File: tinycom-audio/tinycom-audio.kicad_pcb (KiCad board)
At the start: 2 copper layers, 45.2 x 45.2 mm, 73 parts, among them J1 MICRO_SD_HINGE, P1 CONN_02X10, P2 CONN_02X10, P4 USB_OTG, U1 SY8008BAAC, U2 AXP209, U3 SY8008BAAC, U4 RTL8188, U5 rainsun-antenna, U6 admp411, U7 admp411

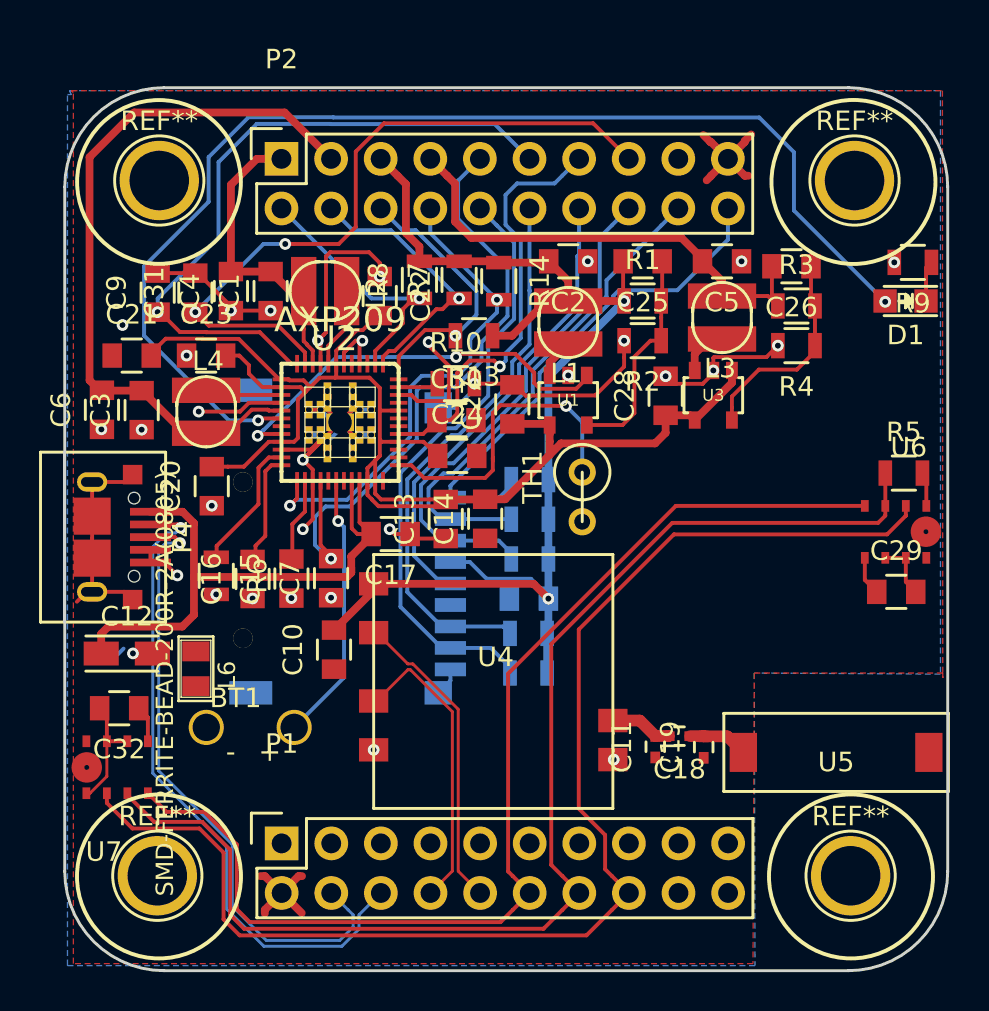
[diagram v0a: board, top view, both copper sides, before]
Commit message: update audio
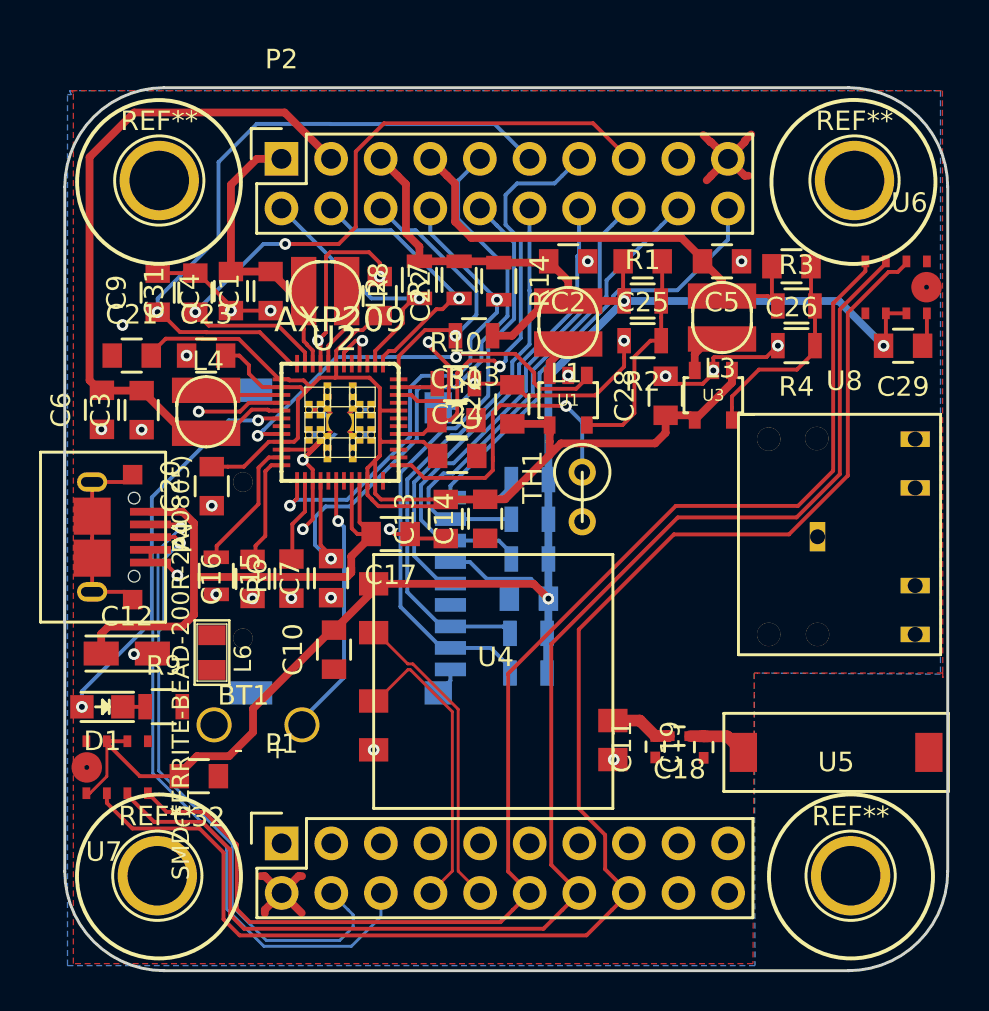
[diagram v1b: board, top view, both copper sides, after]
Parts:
- removed R5: 100K, Resistors_SMD:R_0805
- added U8: audio-jack, tinycom:audio-jack, F.Cu at (165.1, 102.9)
- moved D1 46.1 mm to (126.4, 111.0)
- moved R9 44.6 mm to (129.5, 110.9), turned to 0 degrees
- moved C29 12.6 mm to (167.4, 92.5), turned to 180 degrees
- moved U6 12.5 mm to (167.2, 89.4)
- moved C32 5.36 mm to (131.3, 114.5)
- moved L6 1.17 mm to (132.0, 108.2)
- moved BT1 0.42 mm to (134.4, 111.9)
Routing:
- net Net-(D1-Pad2): track 60.6 -> 20.5 mm
- net VCC_33: track 72.9 -> 101.4 mm, vias 2 -> 3
- net I2S_SCK: track 58.4 -> 68.9 mm
- net I2S_WS: track 67.3 -> 76.9 mm
- net I2S_SD: track 64.1 -> 72.4 mm
- net GND: track 105.5 -> 101.6 mm, vias 31 -> 30
- net (no net): track 1.32 -> 0.00 mm
- net Net-(D1-Pad1): track 2.09 -> 1.15 mm
- net Net-(L6-Pad1): track 11.1 -> 10.4 mm
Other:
- net class Power: trace_width 0.2 -> 0.4
